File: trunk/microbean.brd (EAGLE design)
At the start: 43.2 x 32.7 mm, 17 parts, among them IC2 MAX485ST3485, IC3 PIC16F1827SO

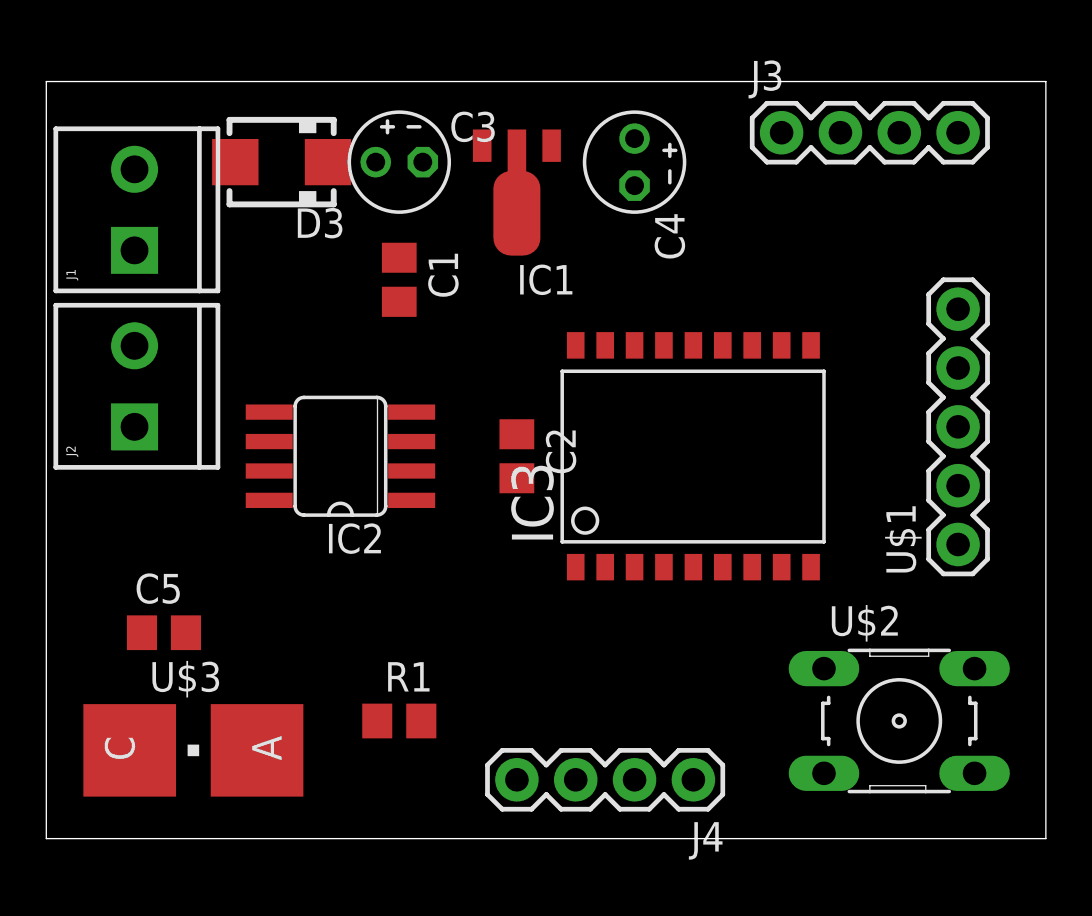
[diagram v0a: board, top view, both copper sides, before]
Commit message: - WIP
git-svn-id: svn://192.168.1.40/net/microbean@535 1a6b750e-079f-425f-90e7-3a118970be6b
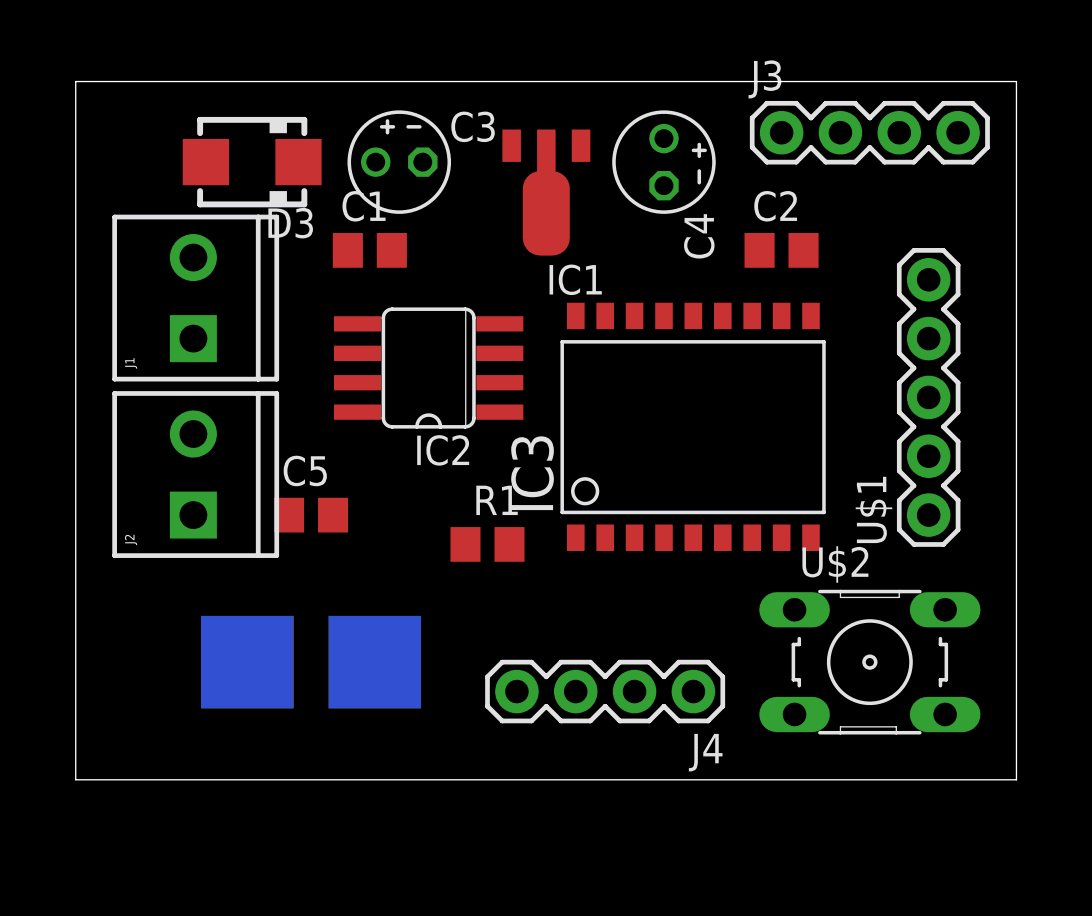
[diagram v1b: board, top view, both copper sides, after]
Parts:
- moved C2 14.5 mm to (31.8, 31.8), turned to 0 degrees
- moved R1 8.52 mm to (19.1, 19.1)
- moved C5 8.13 mm to (11.4, 20.3)
- moved U$3 6.35 mm to (11.4, 14.0), flipped to the bottom, turned to 90 degrees
- moved IC2 5.39 mm to (16.5, 26.7)
- moved J1 4.58 mm to (6.35, 27.9)
- moved J2 4.58 mm to (6.35, 20.3)
- moved J4 3.81 mm to (27.9, 12.7)
- moved U$2 2.84 mm to (35.6, 14.0)
- moved C1 1.80 mm to (14.0, 31.8), turned to 0 degrees
- moved U$1 1.80 mm to (38.1, 20.3)
- moved C4 1.27 mm to (26.7, 35.6)
- moved D3 1.27 mm to (8.89, 35.6)
- moved IC1 1.27 mm to (21.6, 34.3)
- moved IC3 1.27 mm to (27.9, 24.1)
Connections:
- removed net N$4: C2.1, C4.+, IC1.1, IC3.14, U$1.2
- new net N$23: IC2.2, IC2.3, IC3.18
- net N$12: no longer IC2.2, IC2.3, IC3.18
- net N$13: now also C2.1, C4.+, IC1.1, IC3.14, U$1.2
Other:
- board size 43.2 x 32.7 mm -> 40.6 x 30.1 mm

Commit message: WIP
git-svn-id: svn://192.168.1.40/net/microbean@537 1a6b750e-079f-425f-90e7-3a118970be6b
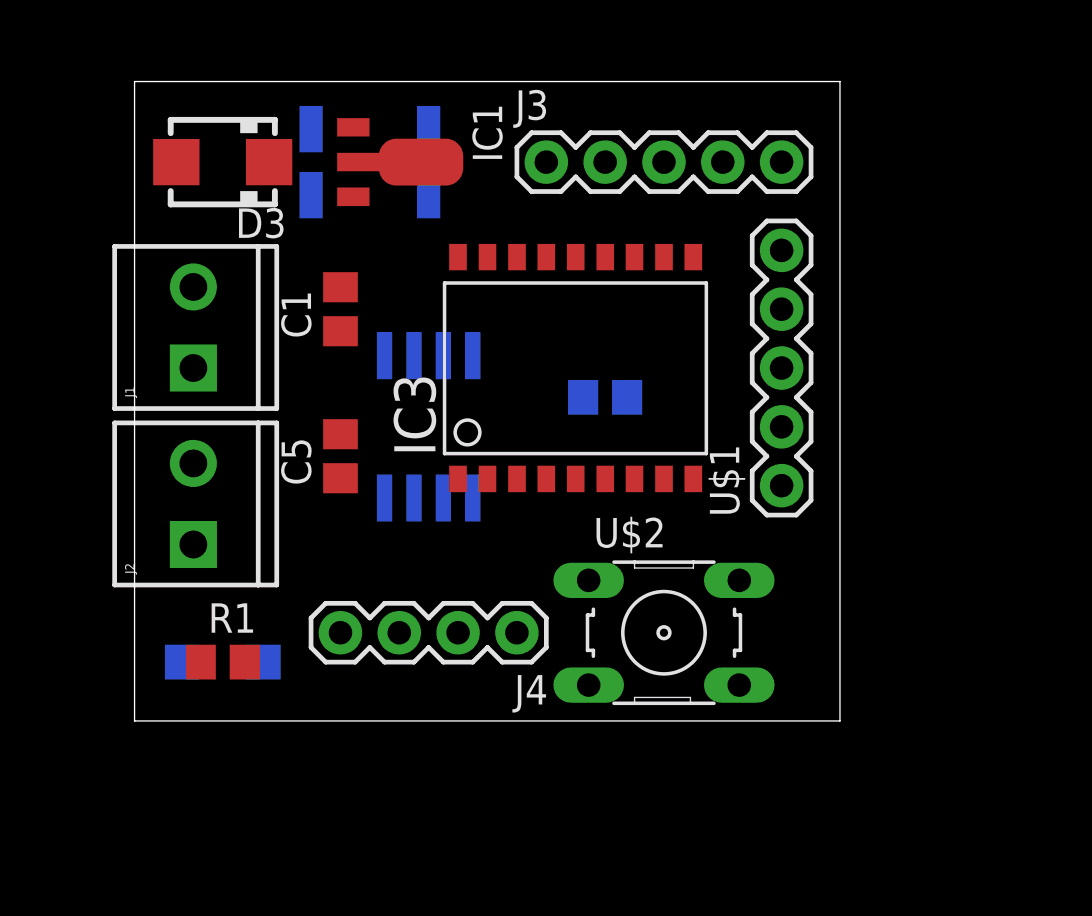
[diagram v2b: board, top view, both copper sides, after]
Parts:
- C3, C4: device custom:E2-4 -> custom:UD-4X5,8_NICHICON
- J3: device custom:1X04 -> custom:1X05
- U$3: value LEDPLCC2 -> LED1206; device custom:P-LCC-2 -> custom:CHIPLED_1206
- moved R1 12.5 mm to (7.62, 14.0)
- moved J3 10.2 mm to (21.6, 35.6)
- moved C4 10.2 mm to (16.5, 35.6), flipped to the bottom, turned to 90 degrees
- moved C2 9.92 mm to (24.1, 25.4), flipped to the bottom
- moved U$2 8.98 mm to (26.7, 15.2)
- moved J4 8.03 mm to (20.3, 15.2)
- moved U$1 6.48 mm to (31.8, 21.6)
- moved IC1 6.48 mm to (15.2, 35.6), turned to 270 degrees
- moved IC3 5.68 mm to (22.9, 26.7)
- moved C3 3.81 mm to (11.4, 35.6), flipped to the bottom, turned to 270 degrees
- moved U$3 3.81 mm to (7.62, 14.0)
- moved C1 2.84 mm to (12.7, 29.2), turned to 90 degrees
- moved C5 2.84 mm to (12.7, 22.9), turned to 90 degrees
- moved IC2 2.54 mm to (16.5, 24.1), flipped to the bottom, turned to 180 degrees
- moved D3 1.27 mm to (7.62, 35.6)
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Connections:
- new net N$4: IC3.16, J3.2
- net N$18: now also J3.5; no longer J3.4
- net N$19: now also J3.4; no longer J3.3
- net N$20: now also J3.3; no longer J3.2
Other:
- board size 40.6 x 30.1 mm -> 30.5 x 27.6 mm
